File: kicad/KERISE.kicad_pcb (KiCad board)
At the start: 2 copper layers, 40.5 x 38.8 mm, 90 parts, among them J1 Host, J10 Host, J11 Slave, J12 Host, J13 Slave, J14 Motor_L, J15 Motor_R, J2 Slave, J3 Host, J4 Slave, J5 ENC_Host, J6 ENC_Slave, J7 ENC_Host, J8 ENC_Slave, J9 COM, P1 ToF_Host, P2 ToF_Slave, Q1 DMN3065LW-7, Q2 DMN3065LW-7, Q3 SFH3015FA, Q4 DMN3065LW-7, Q5 SFH3015FA, Q6 DMN3065LW-7, Q7 SFH3015FA, Q8 DMN3065LW-7, Q9 SFH3015FA, SW1 RESET, SW2 UPLOAD, U1 ESP32-PICO-D4, U2 VL6180X, U3 PCA9632, U4 ICM-20602, U5 MA730, U6 MA730, U7 LXDC2UR30, U8 DRV8835

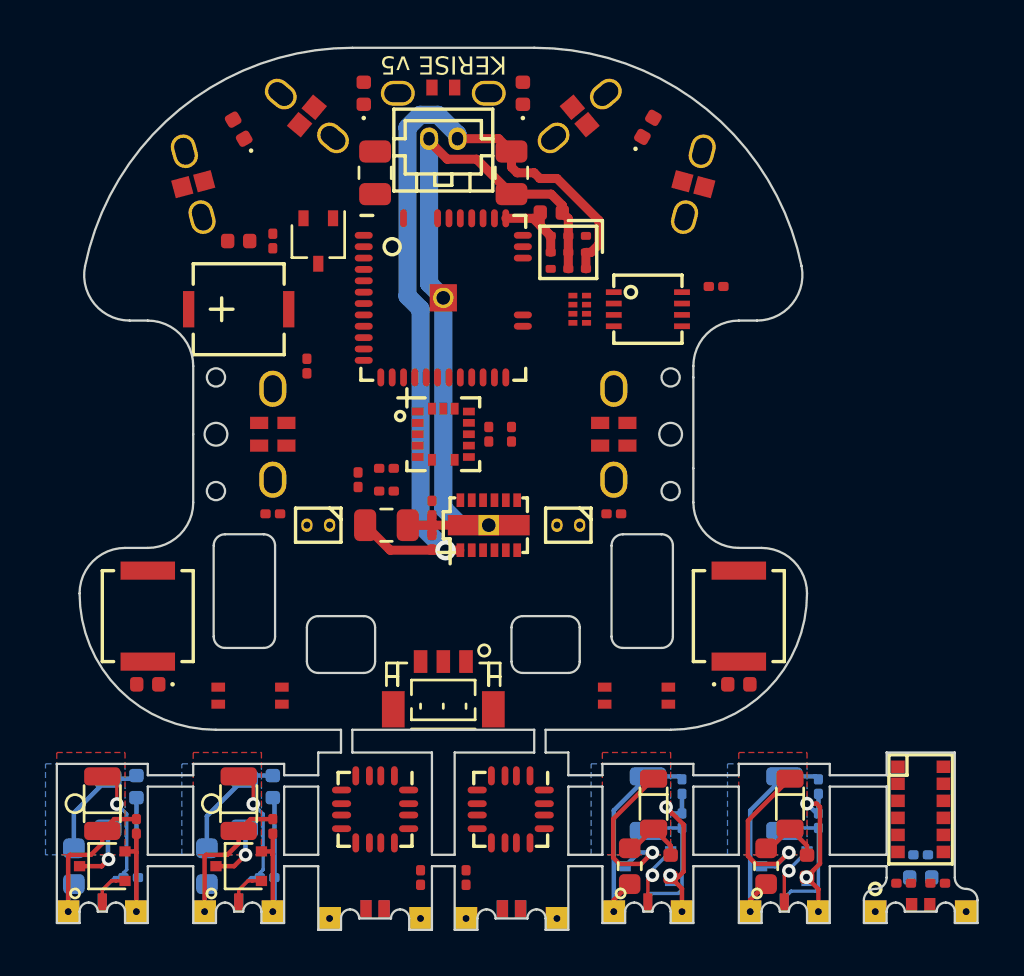
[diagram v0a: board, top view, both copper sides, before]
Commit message: 自動配線完了
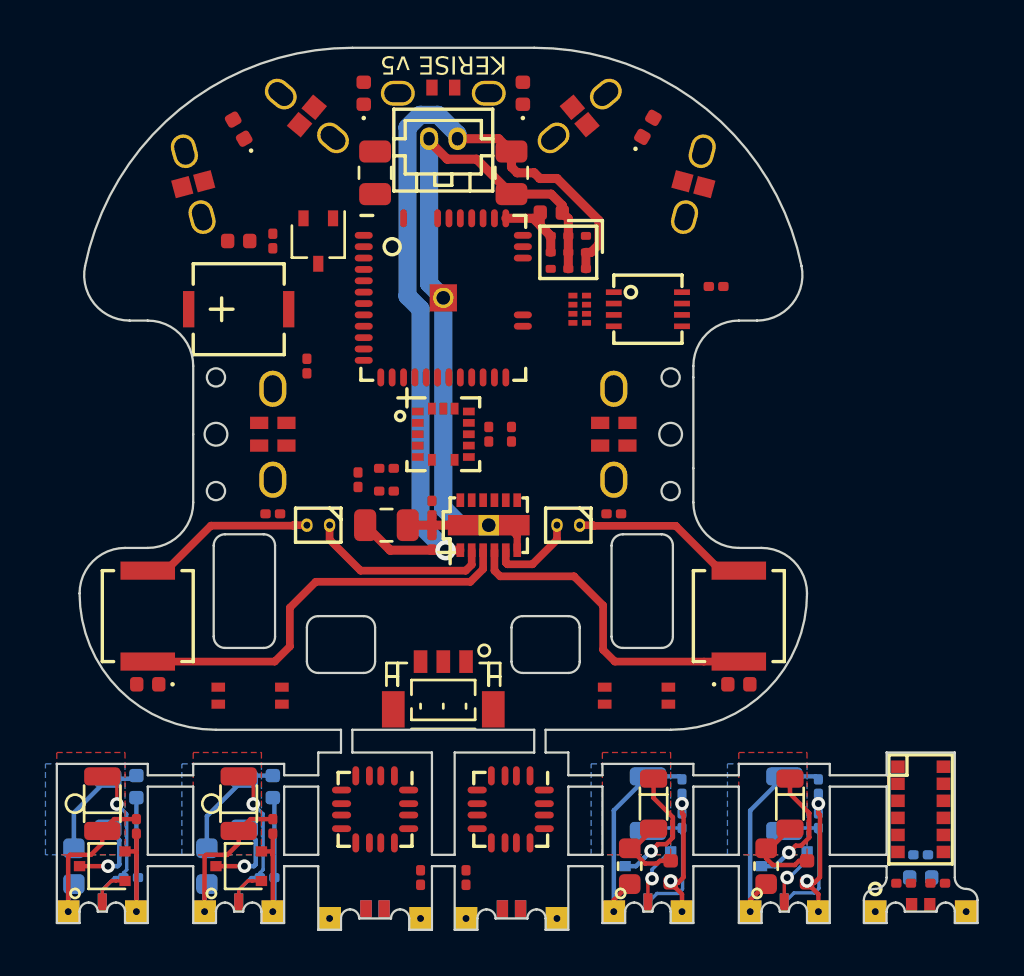
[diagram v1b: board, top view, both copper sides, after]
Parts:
- moved C10 0.25 mm to (164.5, 132.2)
- moved C8 0.25 mm to (158.5, 132.2)
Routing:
- net /Motor/MT_OUT_L_L: track 0.00 -> 18.3 mm
- net /Motor/MT_OUT_L_R: track 0.00 -> 14.4 mm
- net /Motor/MT_OUT_L1: track 0.00 -> 8.20 mm
- net /Motor/MT_OUT_L2: track 0.00 -> 7.83 mm
- net /Motor/MT_OUT_R1: track 0.00 -> 7.83 mm
- net /Motor/MT_OUT_R2: track 0.00 -> 3.91 mm
- net /IR_RCV_FL/LED_to_FET: track 7.77 -> 5.56 mm
- net /IR_RCV_FR/LED_to_FET: track 7.71 -> 5.56 mm
- net GND: track 33.3 -> 35.3 mm
- net /IR_RCV_FR/s_GND: track 7.58 -> 6.35 mm
- net /IR_RCV_FL/s_GND: track 7.41 -> 6.45 mm
- net /IR_RCV_FL/LED_to_C: track 2.88 -> 3.85 mm
- net /IR_RCV_SL/LED_to_FET: track 2.68 -> 3.56 mm
- net /IR_RCV_SR/LED_to_FET: track 2.76 -> 3.56 mm
- net /IR_RCV_FR/LED_to_C: track 2.88 -> 3.53 mm
- added copper zone on F.Cu, net /IR_RCV_FL/LED_to_C
- added copper zone on F.Cu, net /IR_RCV_FR/LED_to_C
- removed copper zone on F.Cu, net /IR_RCV_FL/LED_to_FET
- removed copper zone on F.Cu, net /IR_RCV_FR/LED_to_FET
